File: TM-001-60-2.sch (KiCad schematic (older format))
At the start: 24 parts

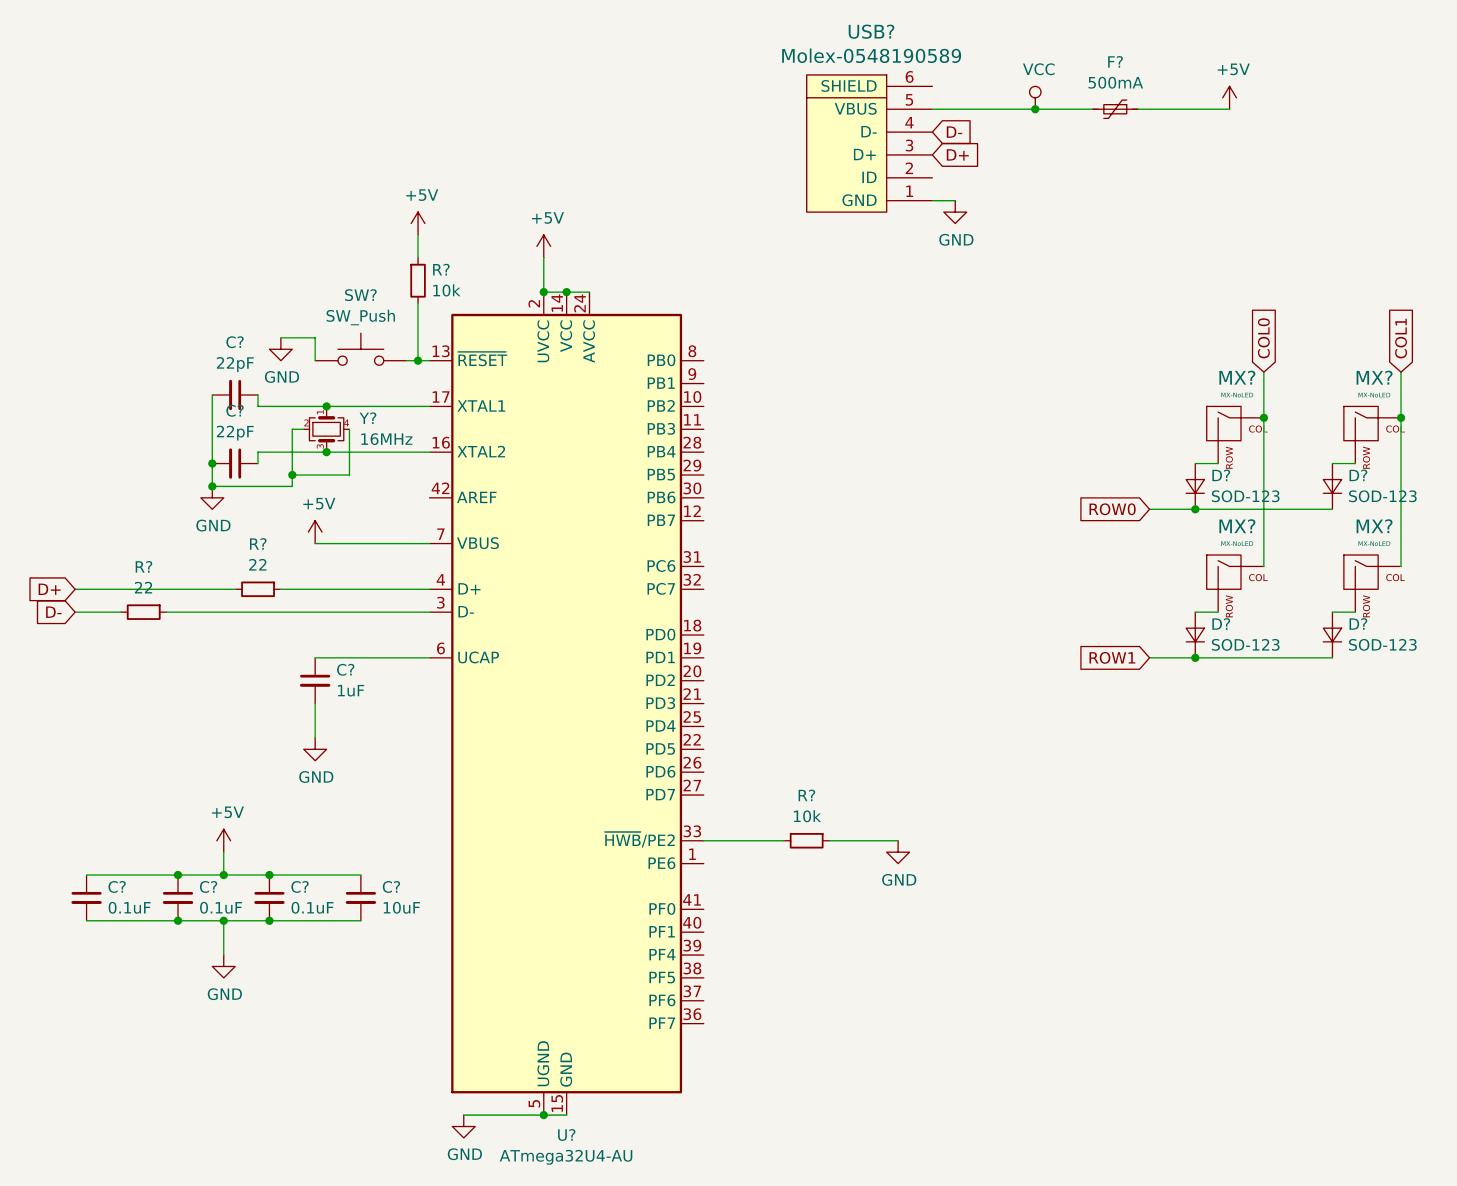
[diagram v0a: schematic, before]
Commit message: ready to create pcb
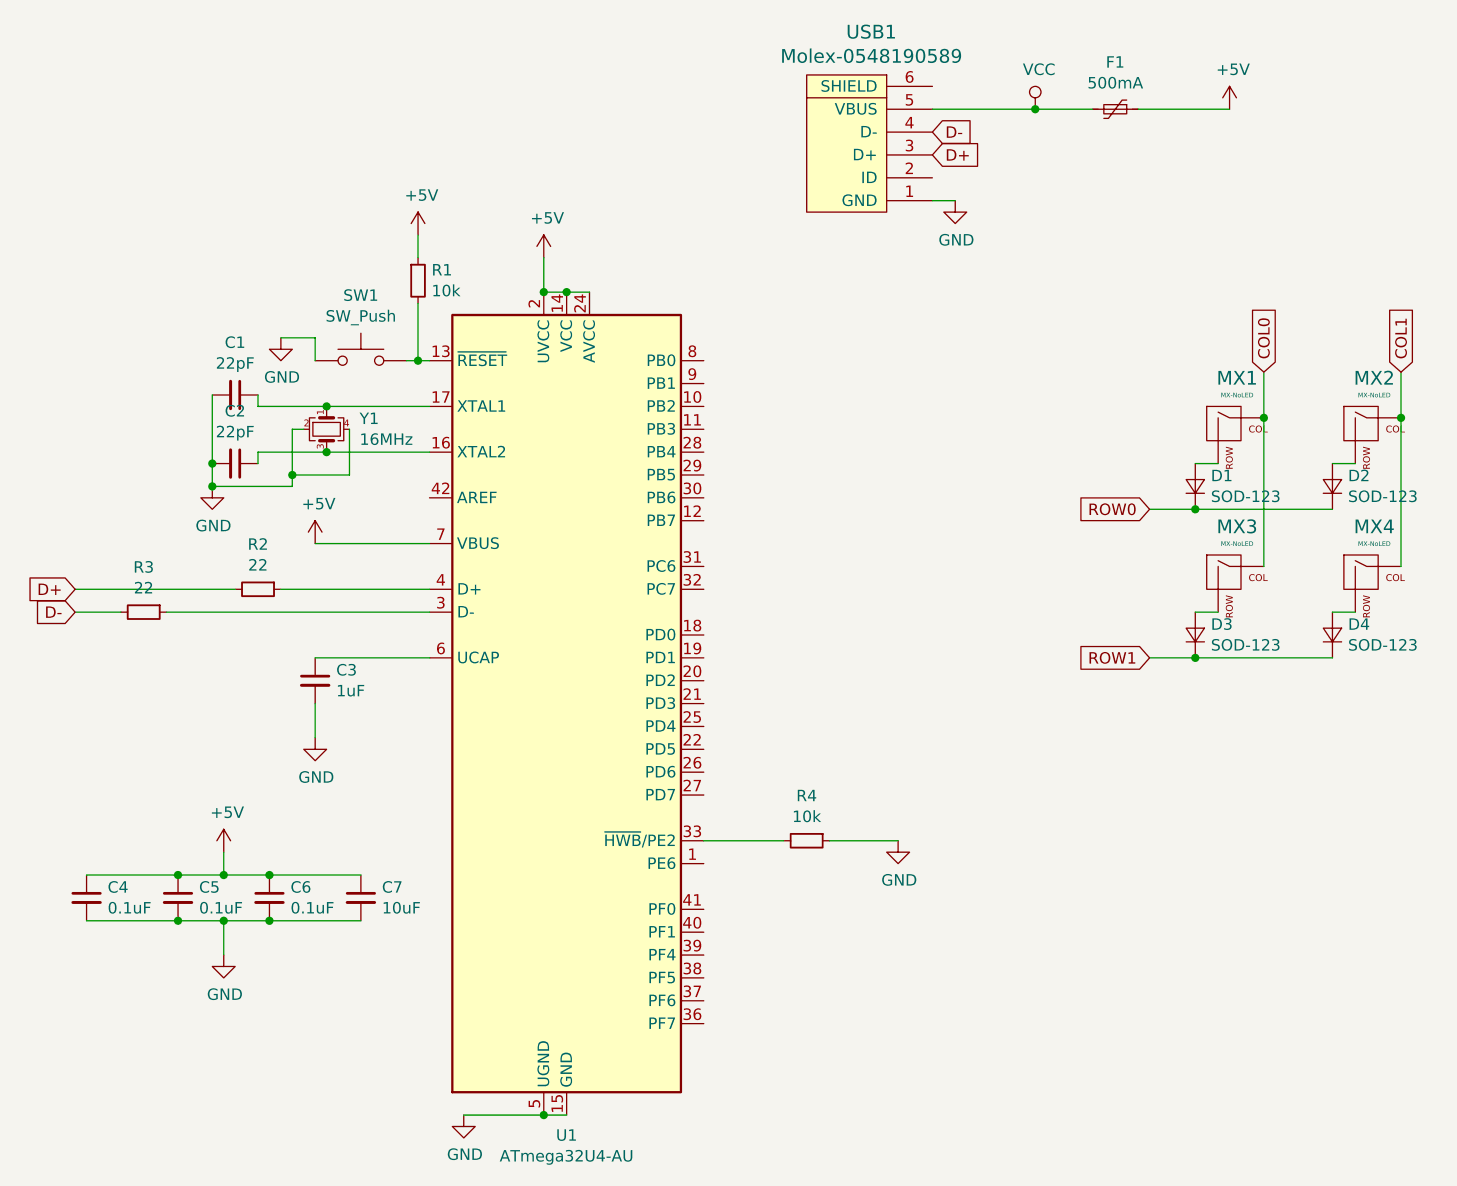
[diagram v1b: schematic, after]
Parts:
- C1, C2, C3, C4, C5, C6, C7: renamed from C?; footprint (none) -> Capacitor_SMD:C_0805_2012Metric
- D1, D2, D3, D4: renamed from D?; footprint (none) -> Diode_SMD:D_SOD-123
- F1: renamed from F?; footprint (none) -> Fuse:Fuse_1206_3216Metric
- MX1, MX2, MX3, MX4: renamed from MX?; footprint (none) -> MX_Alps_Hybrid:MX-1U-NoLED
- SW1: renamed from SW?; footprint (none) -> random-keyboard-parts:SKQG-1155865
- USB1: renamed from USB?; footprint (none) -> random-keyboard-parts:Molex-0548190589
- Y1: renamed from Y?; footprint (none) -> Crystal:Crystal_SMD_3225-4Pin_3.2x2.5mm
- gave numbers to parts that had none: 5

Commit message: fixed footprint assigning
i forgor resistors
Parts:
- R1, R2, R3, R4: footprint (none) -> Resistor_SMD:R_0805_2012Metric
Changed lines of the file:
@@
 F 0 "R4" V 4504 4600 50  0000 C CNN
 F 1 "10k" V 4595 4600 50  0000 C CNN
-F 2 "" H 4700 4600 50  0001 C CNN
+F 2 "Resistor_SMD:R_0805_2012Metric" H 4700 4600 50  0001 C CNN
 F 3 "~" H 4700 4600 50  0001 C CNN
 	1    4700 4600
@@
 F 0 "R2" V 2104 3500 50  0000 C CNN
 F 1 "22" V 2195 3500 50  0000 C CNN
-F 2 "" H 2300 3500 50  0001 C CNN
+F 2 "Resistor_SMD:R_0805_2012Metric" H 2300 3500 50  0001 C CNN
 F 3 "~" H 2300 3500 50  0001 C CNN
 	1    2300 3500
@@
 F 0 "R3" V 1604 3600 50  0000 C CNN
 F 1 "22" V 1695 3600 50  0000 C CNN
-F 2 "" H 1800 3600 50  0001 C CNN
+F 2 "Resistor_SMD:R_0805_2012Metric" H 1800 3600 50  0001 C CNN
 F 3 "~" H 1800 3600 50  0001 C CNN
 	1    1800 3600
@@
 F 0 "R1" H 3059 2196 50  0000 L CNN
 F 1 "10k" H 3059 2105 50  0000 L CNN
-F 2 "" H 3000 2150 50  0001 C CNN
+F 2 "Resistor_SMD:R_0805_2012Metric" H 3000 2150 50  0001 C CNN
 F 3 "~" H 3000 2150 50  0001 C CNN
 	1    3000 2150

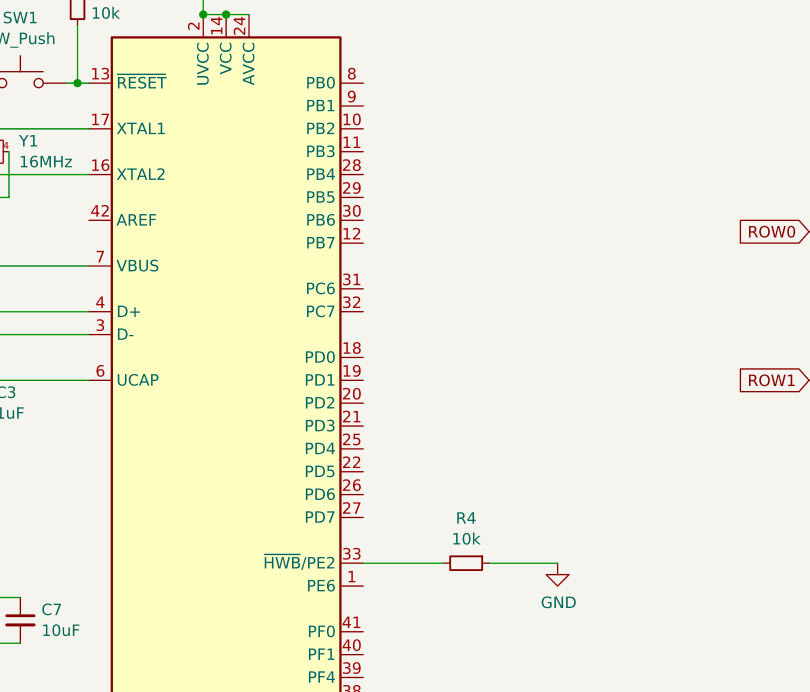
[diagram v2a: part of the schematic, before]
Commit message: saved schematic
i forgor *insert skull emoji*
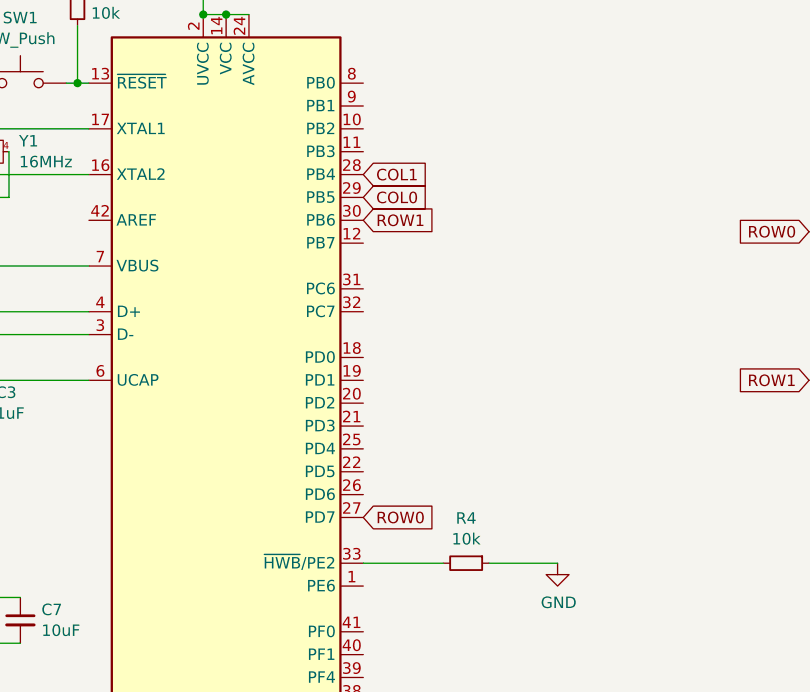
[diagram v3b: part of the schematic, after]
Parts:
- MX1, MX2, MX3, MX4: footprint MX_Alps_Hybrid:MX-1U-NoLED -> MX_Alps_Hybrid:MX-1U
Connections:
- net COL0: now also U1.29 (PB5)
- net COL1: now also U1.28 (PB4)
- net ROW0: now also U1.27 (PD7)
- net ROW1: now also U1.30 (PB6)
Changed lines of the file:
@@
 F 0 "MX1" H 6583 3023 60  0000 C CNN
 F 1 "MX-NoLED" H 6583 2949 20  0000 C CNN
-F 2 "MX_Alps_Hybrid:MX-1U-NoLED" H 5925 2775 60  0001 C CNN
+F 2 "MX_Alps_Hybrid:MX-1U" H 5925 2775 60  0001 C CNN
 F 3 "" H 5925 2775 60  0001 C CNN
 	1    6550 2800
@@
 F 0 "MX2" H 7183 3023 60  0000 C CNN
 F 1 "MX-NoLED" H 7183 2949 20  0000 C CNN
-F 2 "MX_Alps_Hybrid:MX-1U-NoLED" H 6525 2775 60  0001 C CNN
+F 2 "MX_Alps_Hybrid:MX-1U" H 6525 2775 60  0001 C CNN
 F 3 "" H 6525 2775 60  0001 C CNN
 	1    7150 2800
@@
 F 0 "MX3" H 6583 3673 60  0000 C CNN
 F 1 "MX-NoLED" H 6583 3599 20  0000 C CNN
-F 2 "MX_Alps_Hybrid:MX-1U-NoLED" H 5925 3425 60  0001 C CNN
+F 2 "MX_Alps_Hybrid:MX-1U" H 5925 3425 60  0001 C CNN
 F 3 "" H 5925 3425 60  0001 C CNN
 	1    6550 3450
@@
 F 0 "MX4" H 7183 3673 60  0000 C CNN
 F 1 "MX-NoLED" H 7183 3599 20  0000 C CNN
-F 2 "MX_Alps_Hybrid:MX-1U-NoLED" H 6525 3425 60  0001 C CNN
+F 2 "MX_Alps_Hybrid:MX-1U" H 6525 3425 60  0001 C CNN
 F 3 "" H 6525 3425 60  0001 C CNN
 	1    7150 3450
@@
 Text GLabel 7300 2550 1    50   Input ~ 0
 COL1
+Text GLabel 4250 2900 2    50   Input ~ 0
+COL1
+Text GLabel 4250 3000 2    50   Input ~ 0
+COL0
+Text GLabel 4250 3100 2    50   Input ~ 0
+ROW1
+Text GLabel 4250 4400 2    50   Input ~ 0
+ROW0
 $EndSCHEMATC
